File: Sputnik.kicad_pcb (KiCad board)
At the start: 4 copper layers, 130 x 60 mm, 132 parts, among them IC1 EP4CE10F17, J1 Pinheader_2x5_TH_WALL, U1 SN74LVC2T45, U10 SN74LVC8T245, U11 SN74LVC8T245, U12 SN74LVC8T245, U13 SN74LVC8T245, U14 SN74LVC8T245, U15 SN74LVC8T245, U16 SN74LVC2T45, U17 SN74LVC2T45, U18 SN74LVC2T45, U19 SN74LVC1G07DCK, U2 SN74LVC2T45, U20 SN74LVC2T45, U21 EPCS4, U22 W9751G6KB, U23 FT313HL-LQFP64-0.5, U3 SN74LVC1G07DCK, U4 SN74LVC2T45, U5 DM9000B, U6 93LC46, U7 74LVC2G07, U8 Pulse-J00-0045NL, U9 SN74LVC8T245, X2 Zorro_Connector

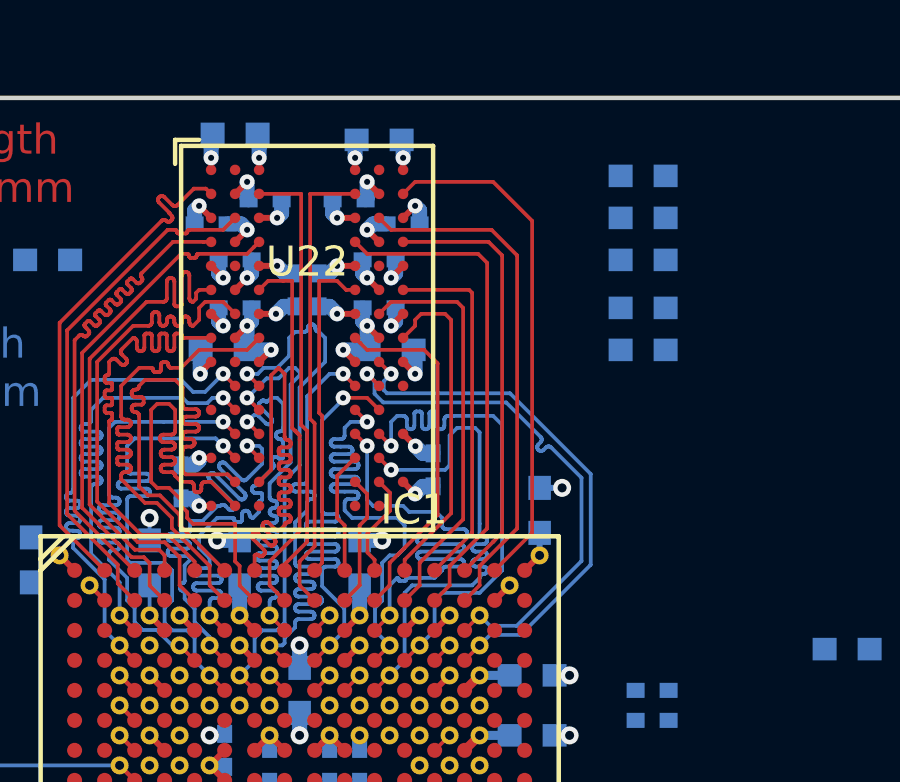
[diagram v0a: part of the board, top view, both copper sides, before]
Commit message: More tuning
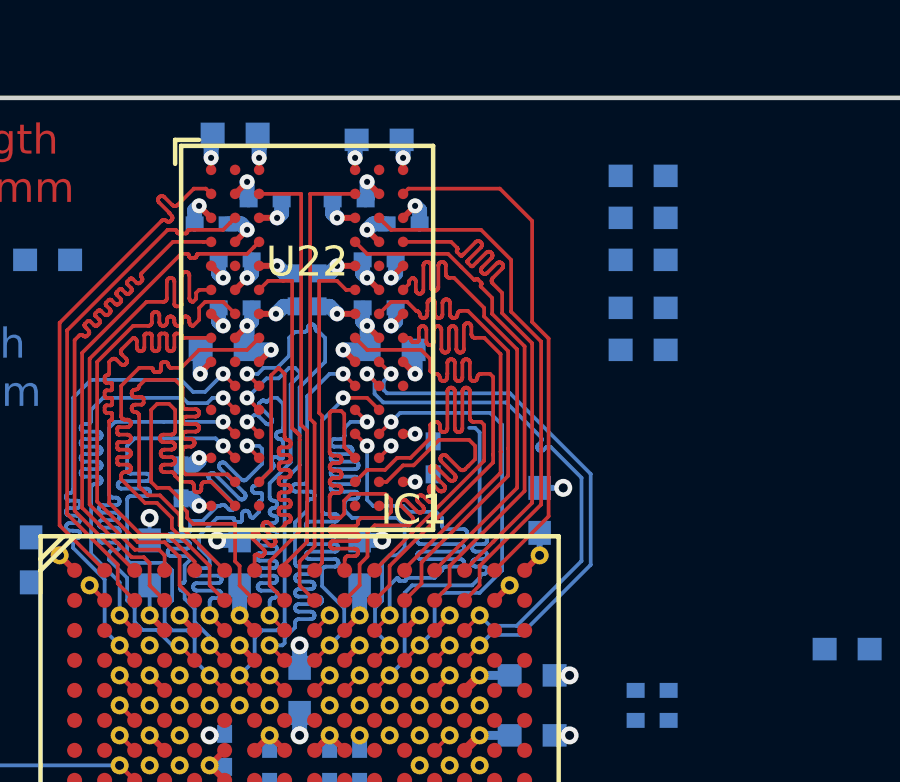
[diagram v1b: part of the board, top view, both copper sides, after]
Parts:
- moved C86 0.40 mm to (188.2, 32.0)
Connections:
- IC1 pad A11: /RAM/A8 -> /RAM/A11
- IC1 pad B10: /RAM/A11 -> /RAM/A8
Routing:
- net /RAM/A8: track 3.51 -> 17.2 mm
- net /RAM/A6: track 4.10 -> 17.2 mm
- net /RAM/A11: track 4.43 -> 17.2 mm
- net /RAM/DQ5: track 11.1 -> 17.2 mm
- net /RAM/DQ2: track 11.9 -> 17.2 mm
- net /RAM/DQ7: track 12.1 -> 17.2 mm
- net /RAM/DQ13: track 14.6 -> 18.6 mm
- net /RAM/A4: track 17.8 -> 14.1 mm
- net /RAM/DQ0: track 13.6 -> 17.2 mm
- net /RAM/A0: track 17.9 -> 14.5 mm
- net +1V8: track 27.8 -> 27.0 mm
- net GND: track 199.0 -> 198.2 mm
- net /RAM/DQ10: track 16.7 -> 17.2 mm

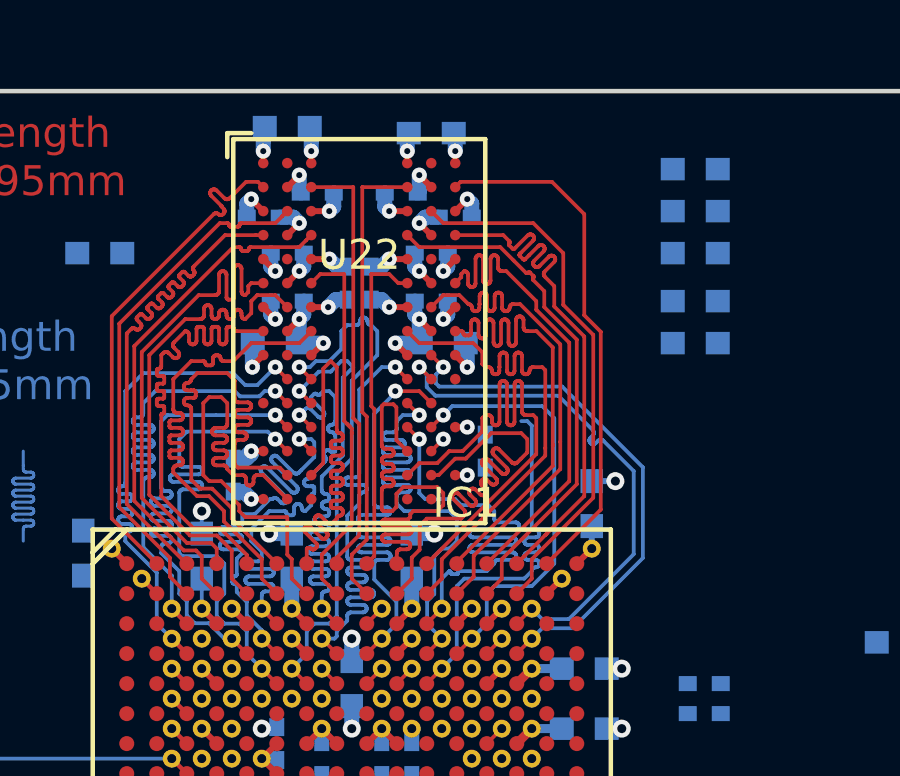
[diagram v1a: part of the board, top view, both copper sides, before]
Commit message: Up
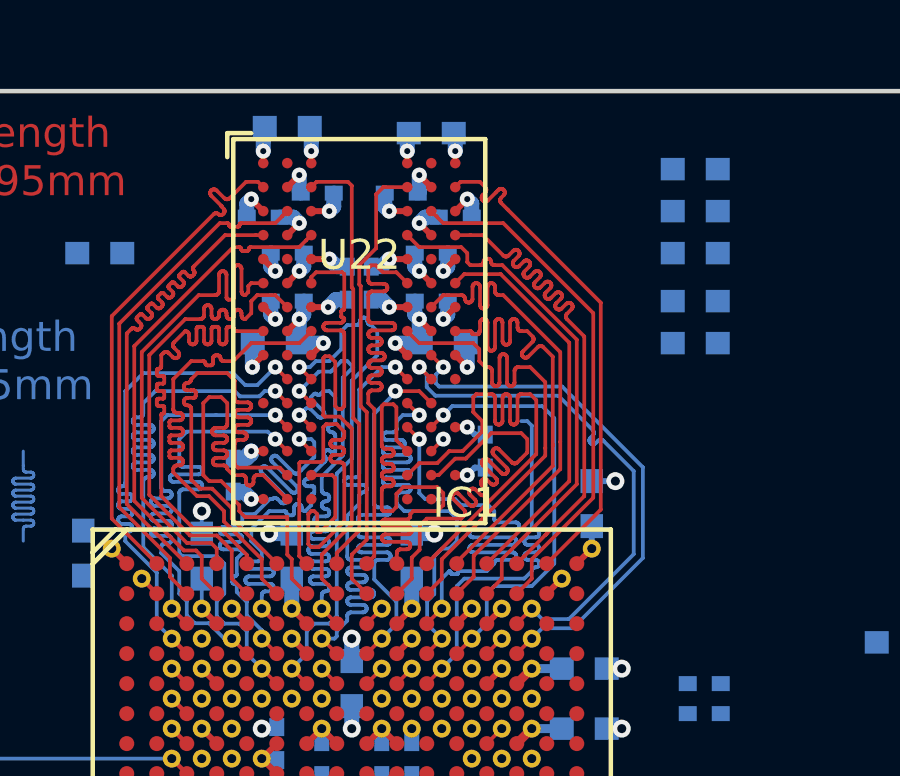
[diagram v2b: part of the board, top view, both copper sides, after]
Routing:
- net /RAM/LDQS: track 11.1 -> 17.2 mm
- net /RAM/LDM: track 12.7 -> 18.7 mm
- net /RAM/DQ7: track 17.2 -> 13.4 mm
- net GND: track 198.2 -> 198.9 mm
- net +1V8: track 27.0 -> 27.7 mm
- net /RAM/DQ8: track 17.8 -> 17.2 mm

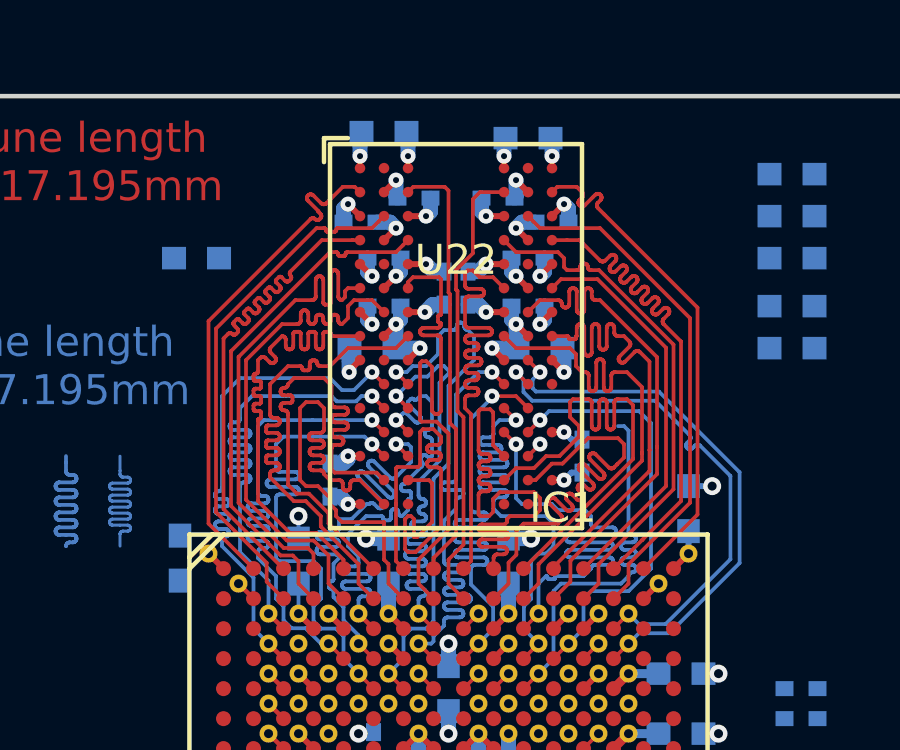
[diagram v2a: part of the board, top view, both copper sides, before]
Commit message: Up..
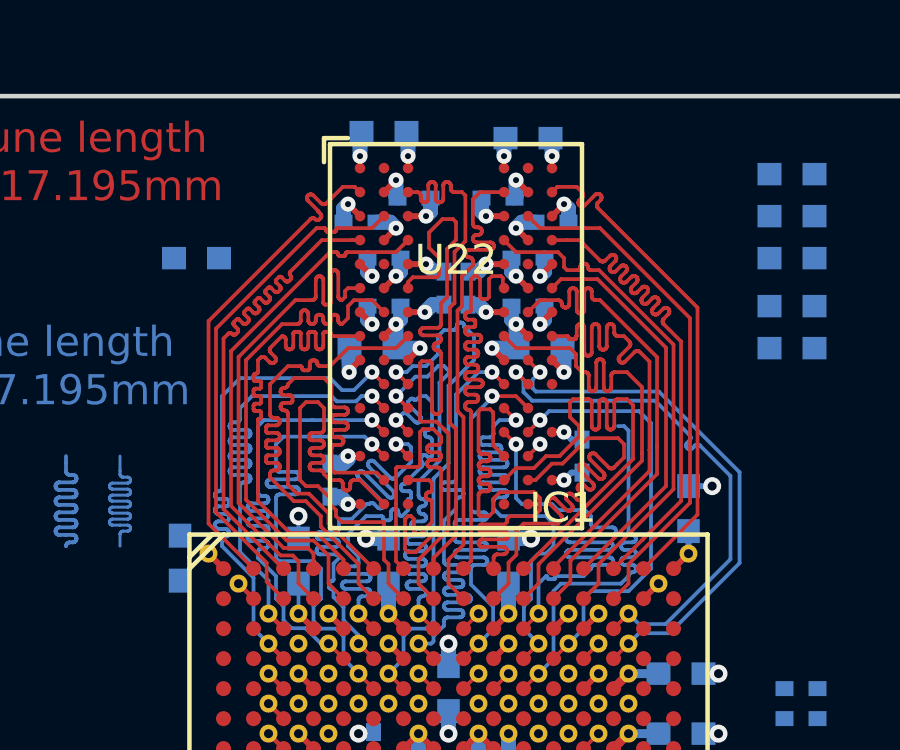
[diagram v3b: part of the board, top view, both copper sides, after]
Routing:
- net /RAM/LDM: track 18.7 -> 23.7 mm
- net /RAM/UDM: track 14.5 -> 17.2 mm
- net /RAM/UDQS: track 15.2 -> 17.1 mm

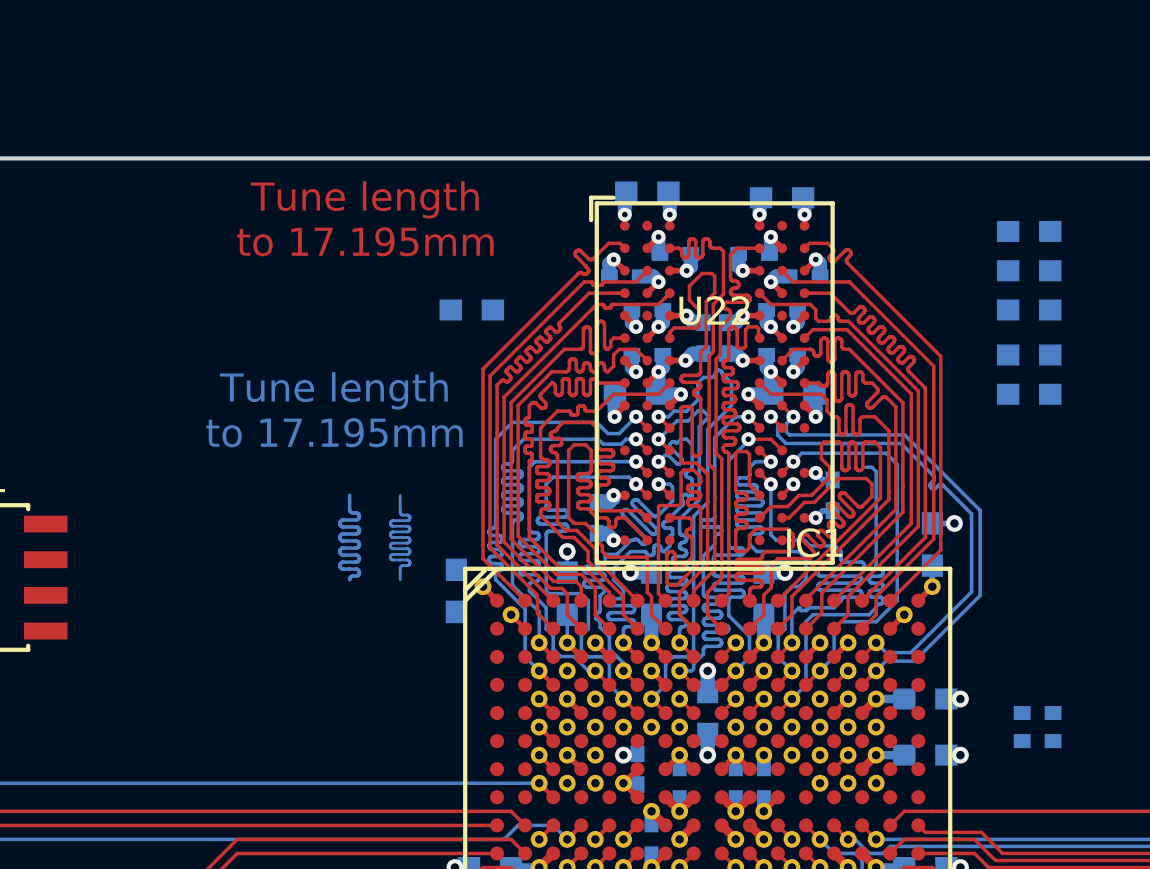
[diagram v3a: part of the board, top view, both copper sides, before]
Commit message: More tuning...
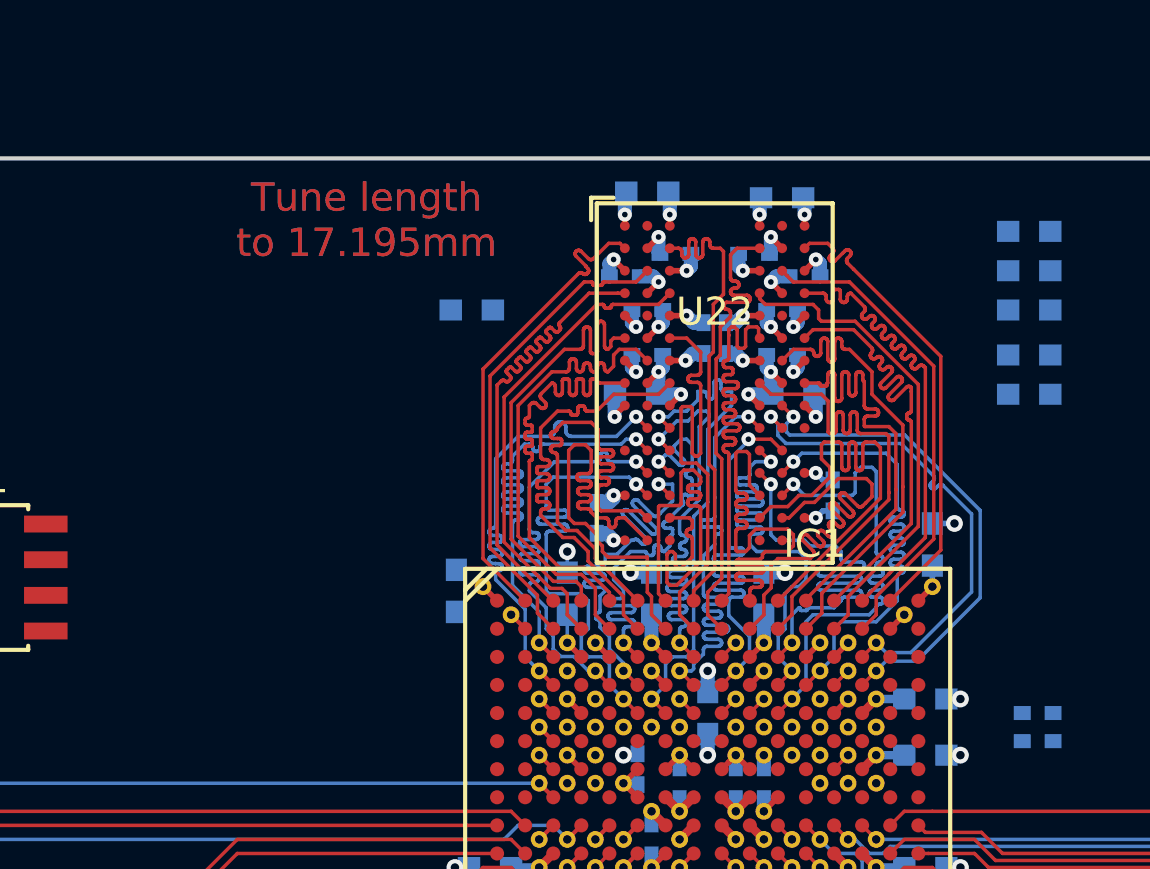
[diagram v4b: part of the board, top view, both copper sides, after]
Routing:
- net (no net): track 16.7 -> 0.00 mm
- net /RAM/LDM: track 23.7 -> 17.2 mm
- net /RAM/A4: track 14.1 -> 17.9 mm
- net /RAM/DQ7: track 13.4 -> 17.2 mm
- net /RAM/A0: track 14.5 -> 17.9 mm
